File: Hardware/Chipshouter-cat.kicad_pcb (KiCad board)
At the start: 2 copper layers, 23.7 x 40.7 mm, 74 parts, among them J1 Antenna, J2 BG306-02-A-2-0400-L-G, J3 Header7, J4 Header 2, J5 Header 4, J6 Input Power:2x AA Battery, P1 USB_C_Plug_USB2.0, Q1 AO3422, Q2 AO3422, Q3 LDA111STR, Q4 RGT16BM65DTL, SW1 TL3301AF160QJ, SW2 ON, SW3 KSC741JLFS, SW4 RESET, SW5 BOOT, SW6 KSC741JLFS, T1 ATB322524, T2 ATB322524, U1 AP2112K-3.3, U2 W25Q16JV, U3 RP2040, Y1 12Mhz

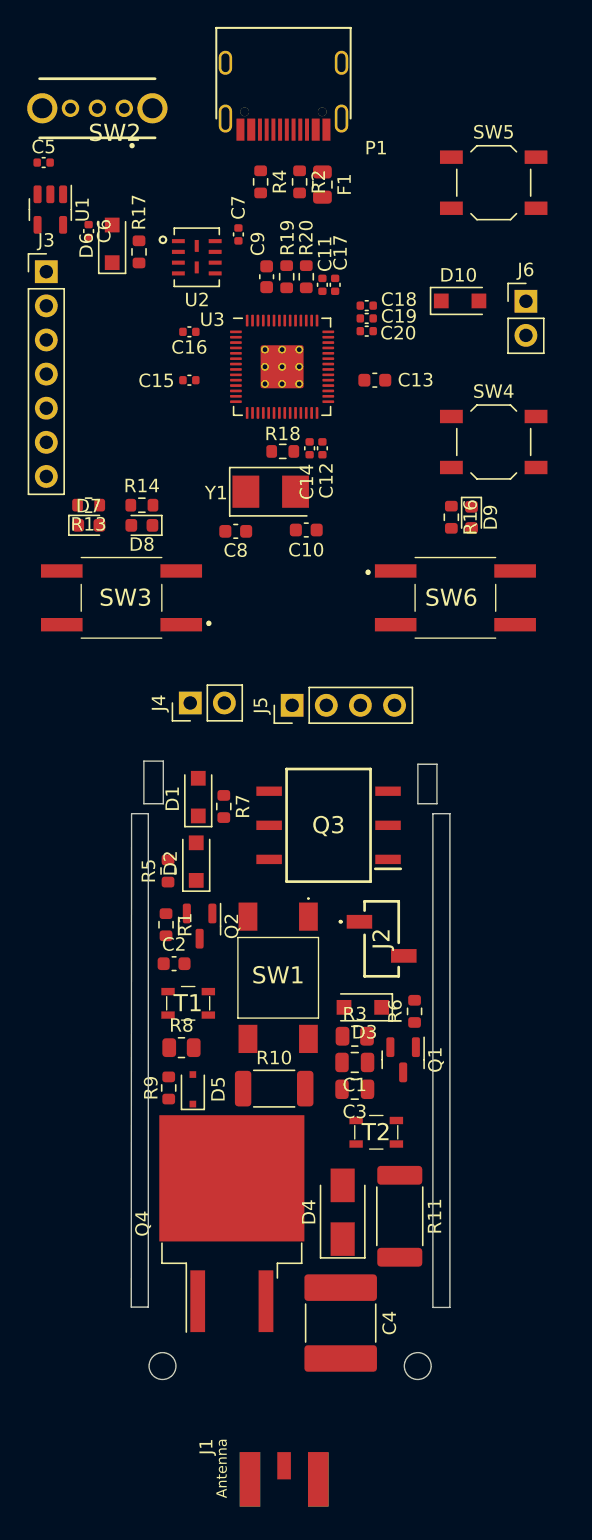
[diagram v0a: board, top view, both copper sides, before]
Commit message: Finished routing
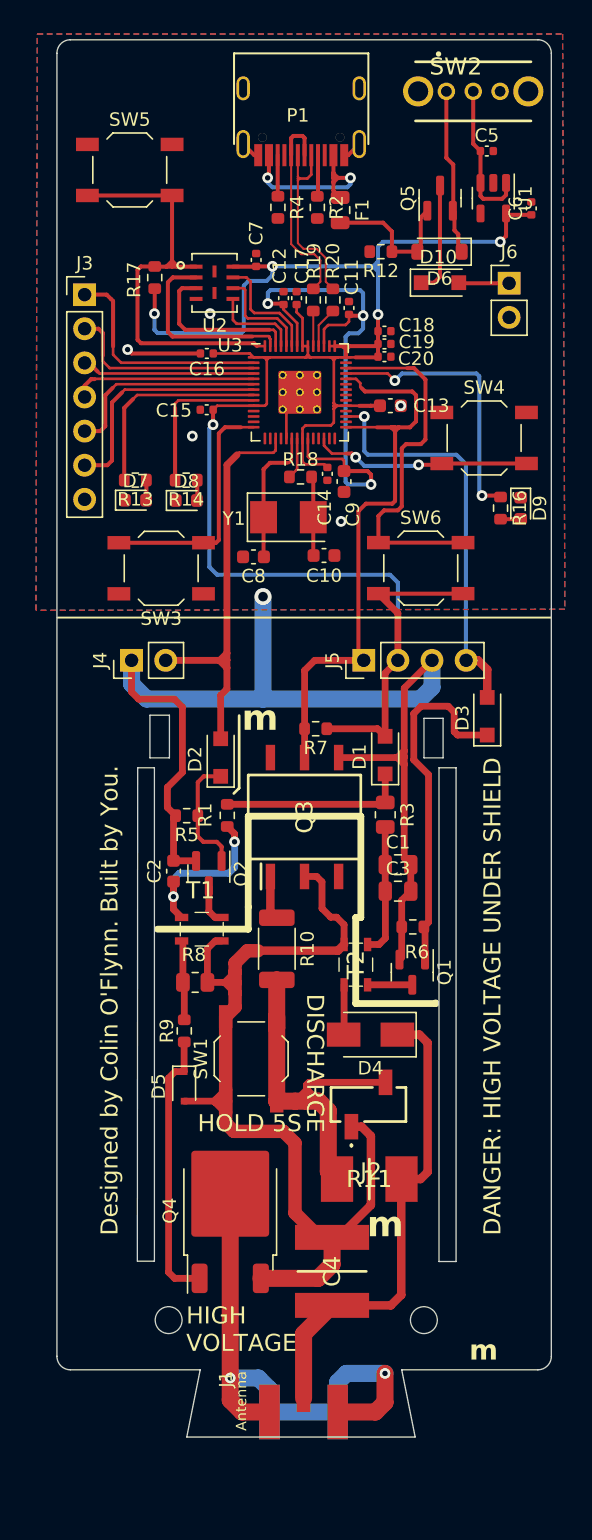
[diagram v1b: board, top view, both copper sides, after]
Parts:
- removed the ? at (74.7, 118.5)
- removed the ? at (55.7, 118.5)
- added ?: , , F.Cu at (56.2, 115.1)
- added ?: , , F.Cu at (75.2, 115.1)
- added Q5: DMG3415U-7, Package_TO_SOT_SMD:SOT-23, F.Cu at (76.4, 31.6)
- added R12: 100K, Resistor_SMD:R_0603_1608Metric, F.Cu at (72.0, 35.6)
- C4: footprint Capacitor_SMD:C_2220_5650Metric_Pad1.97x5.40mm_HandSolder -> chipshouter:CAPC6153X500N
- D6: footprint Diode_SMD:D_SOD-123F -> Diode_SMD:D_SOD-123
- Q4: footprint Package_TO_SOT_SMD:TO-263-2 -> Package_TO_SOT_SMD:TO-252-3_TabPin2
- R11: footprint Resistor_SMD:R_2512_6332Metric_Pad1.40x3.35mm_HandSolder -> chipshouter:RESC6432X120N
- SW1: value TL3301AF160QJ -> TL3342F450QG; footprint chipshouter:TL3301AF160QJ -> Button_Switch_SMD:SW_SPST_TL3342
- SW3, SW6: value KSC741JLFS -> TL3342F450QG; footprint chipshouter:KSC401G50SHLFS -> Button_Switch_SMD:SW_SPST_TL3342
- moved C5 33.0 mm to (79.9, 28.1)
- moved C6 33.0 mm to (83.2, 32.4), turned to 90 degrees
- moved U1 33.0 mm to (80.4, 31.6)
- moved SW2 28.0 mm to (78.9, 23.6), turned to 0 degrees
- moved SW5 27.1 mm to (53.3, 29.5)
- moved D6 24.4 mm to (76.4, 35.6), turned to 180 degrees
- moved D3 23.6 mm to (79.9, 70.2), turned to 90 degrees
- moved R3 16.6 mm to (72.3, 77.5), turned to -90 degrees
- moved C9 16.3 mm to (69.3, 52.7), turned to -90 degrees
- moved C3 15.1 mm to (73.3, 83.2), turned to 0 degrees
- moved C1 15.1 mm to (73.3, 81.2), turned to 0 degrees
- moved D1 14.3 mm to (72.3, 73.1)
- moved D4 13.4 mm to (71.2, 93.9), turned to 180 degrees
- moved T2 12.6 mm to (70.1, 88.7), turned to 90 degrees
- moved J2 12.4 mm to (71.1, 99.1), turned to 0 degrees
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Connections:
- net Net-(R19-Pad2) renamed /+
- net Net-(R20-Pad2) renamed /-
- C6 pad 1: Net-(C6-Pad1) -> +3V3
- D1 pad 2: VCC -> +3V3
- D10 pad 1: +3V3 -> /VSYS
- D6 pad 1: +3V3 -> Net-(D6-K)
- D6 pad 2: Net-(C6-Pad1) -> VBUS
- J5 pad 2: VCC -> +3V3
- R7 pad 1: VCC -> +3V3
- SW2 pad 1: VBUS -> Net-(D6-K)
- SW6 pad 2: VCC -> +3V3
- U1 pad 5: Net-(C6-Pad1) -> +3V3
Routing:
- net +3V3: track 0.00 -> 151.9 mm, vias 0 -> 5
- net GND: track 0.00 -> 96.0 mm, vias 0 -> 6
- net Net-(D5-A): track 0.00 -> 74.6 mm
- net /CHARGED: track 0.00 -> 45.0 mm
- net +1V2: track 0.00 -> 42.3 mm, vias 0 -> 3
- net Net-(J1-Ext): track 0.00 -> 40.7 mm, vias 0 -> 2
- net Net-(D4-K): track 0.00 -> 36.2 mm
- net /QSPI_CS: track 0.00 -> 32.2 mm
- net /GP14: track 0.00 -> 31.7 mm
- net /GP20: track 0.00 -> 30.5 mm, vias 0 -> 1
- net Net-(J2-Pin_2): track 0.00 -> 29.1 mm
- net /GP28: track 0.00 -> 27.4 mm
- net Net-(D3-K): track 0.00 -> 26.4 mm
- net /GP27: track 0.00 -> 20.8 mm, vias 0 -> 2
- net Net-(D5-K): track 0.00 -> 20.5 mm
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- added copper zone on B.Cu, net GND
- added copper zone on F.Cu, net GND
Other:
- board size 23.7 x 40.7 mm -> 36.8 x 104 mm
- board text added: "DANGER: HIGH VOLTAGE UNDER SHIELD"
- board text added: "DISCHARGE"
- board text added: "Designed by Colin O'Flynn. Built by You."
- board text added: "HIGH VOLTAGE"
- board text added: "HOLD 5S"
- board text added: "m"
